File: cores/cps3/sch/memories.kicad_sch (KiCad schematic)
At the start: 2 parts, among them K12 29F016-90PFTN

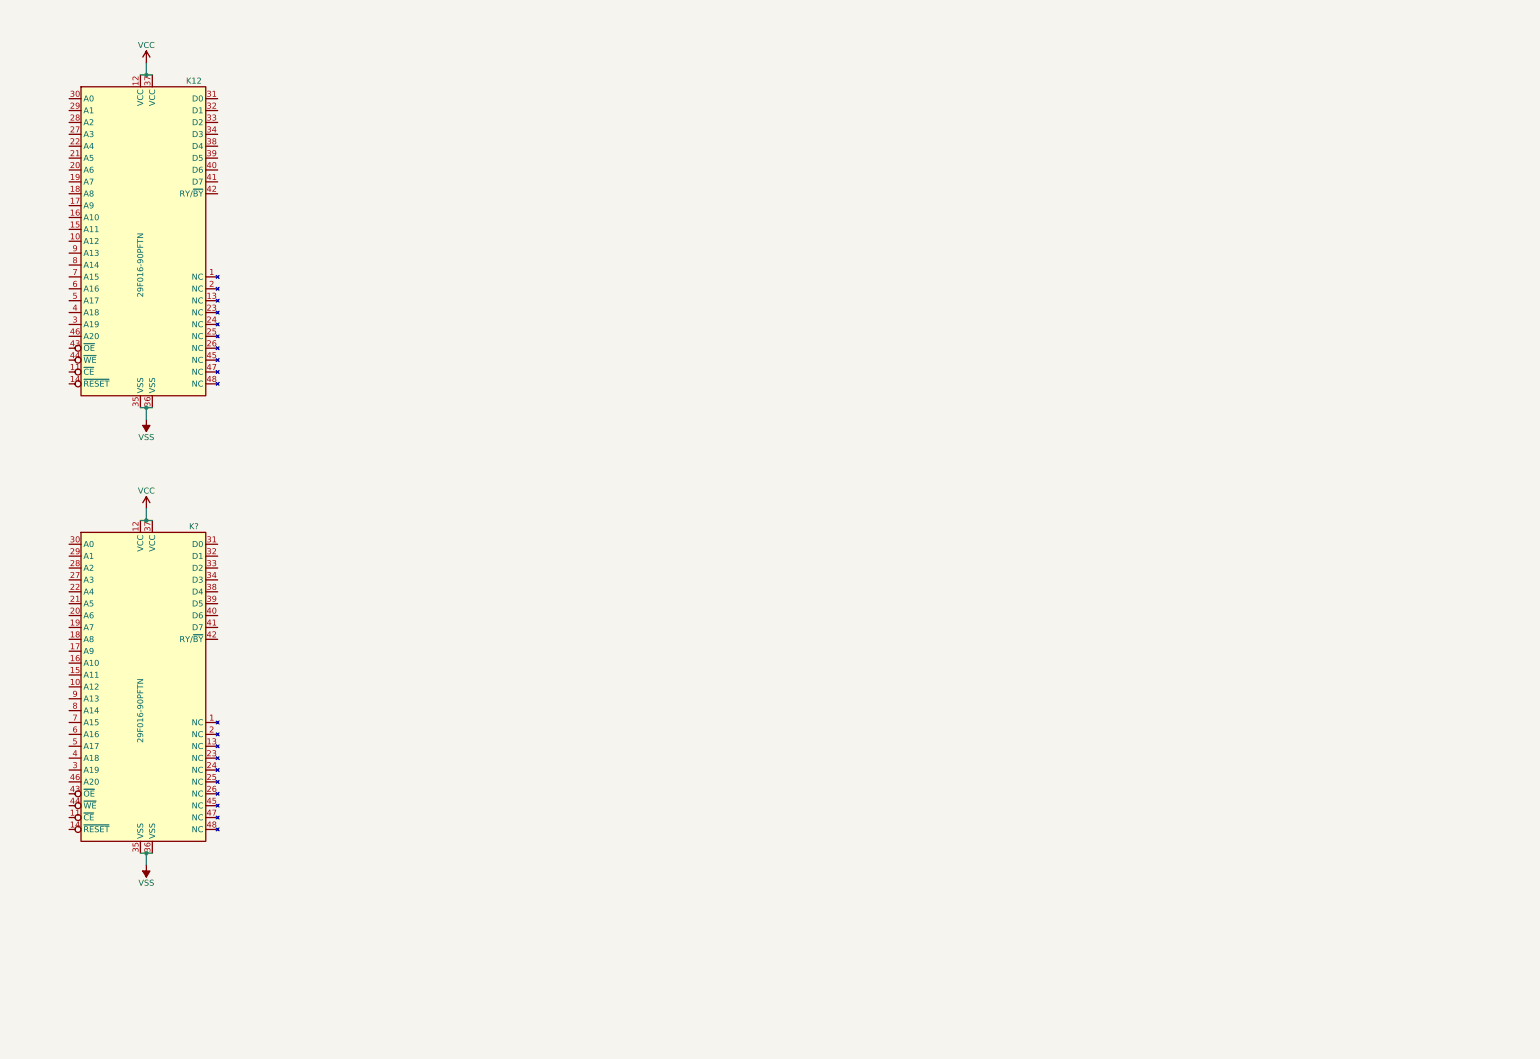
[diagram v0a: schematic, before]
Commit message: memories_gfx_main
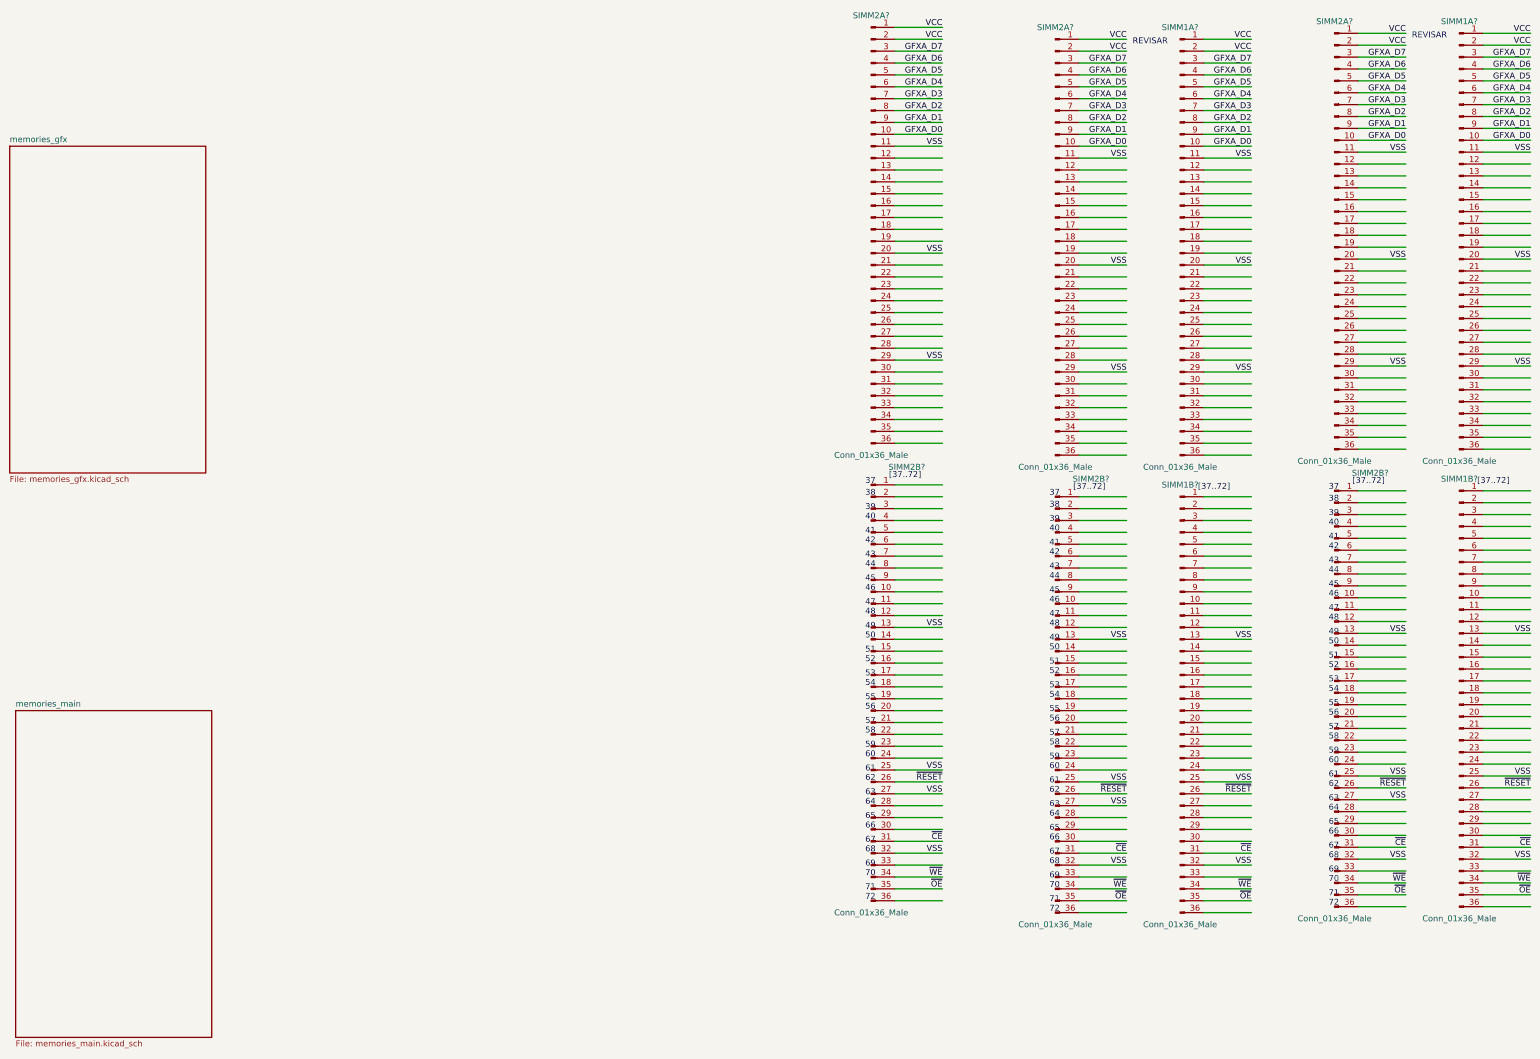
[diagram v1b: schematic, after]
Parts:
- removed K12, K?: 29F016-90PFTN, symbol arcade:29F016-90PFTN
- added SIMM1A? (x2), SIMM1B? (x2), SIMM2A? (x3), SIMM2B? (x3): Conn_01x36_Male, symbol Connector:Conn_01x36_Male
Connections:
- net VCC: now also SIMM1A?.1 (Pin_1), SIMM1A?.1 (Pin_1), SIMM1A?.2 (Pin_2), SIMM1A?.2 (Pin_2), SIMM2A?.1 (Pin_1), SIMM2A?.1 (Pin_1), SIMM2A?.1 (Pin_1), SIMM2A?.2 (Pin_2), SIMM2A?.2 (Pin_2), SIMM2A?.2 (Pin_2)
- net VSS: now also SIMM1A?.11 (Pin_11), SIMM1A?.11 (Pin_11), SIMM1A?.20 (Pin_20), SIMM1A?.20 (Pin_20), SIMM1A?.29 (Pin_29), SIMM1A?.29 (Pin_29), SIMM1B?.13 (Pin_13), SIMM1B?.13 (Pin_13), SIMM1B?.25 (Pin_25), SIMM1B?.25 (Pin_25), SIMM1B?.32 (Pin_32), SIMM1B?.32 (Pin_32), SIMM2A?.11 (Pin_11), SIMM2A?.11 (Pin_11), SIMM2A?.11 (Pin_11), SIMM2A?.20 (Pin_20), SIMM2A?.20 (Pin_20), SIMM2A?.20 (Pin_20), SIMM2A?.29 (Pin_29), SIMM2A?.29 (Pin_29), SIMM2A?.29 (Pin_29), SIMM2B?.13 (Pin_13), SIMM2B?.13 (Pin_13), SIMM2B?.13 (Pin_13), SIMM2B?.25 (Pin_25), SIMM2B?.25 (Pin_25), SIMM2B?.25 (Pin_25), SIMM2B?.27 (Pin_27), SIMM2B?.27 (Pin_27), SIMM2B?.27 (Pin_27), SIMM2B?.32 (Pin_32), SIMM2B?.32 (Pin_32), SIMM2B?.32 (Pin_32)
- new net GFXA_D0: SIMM1A?.10 (Pin_10), SIMM1A?.10 (Pin_10), SIMM2A?.10 (Pin_10), SIMM2A?.10 (Pin_10), SIMM2A?.10 (Pin_10)
- new net GFXA_D1: SIMM1A?.9 (Pin_9), SIMM1A?.9 (Pin_9), SIMM2A?.9 (Pin_9), SIMM2A?.9 (Pin_9), SIMM2A?.9 (Pin_9)
- new net GFXA_D2: SIMM1A?.8 (Pin_8), SIMM1A?.8 (Pin_8), SIMM2A?.8 (Pin_8), SIMM2A?.8 (Pin_8), SIMM2A?.8 (Pin_8)
- new net GFXA_D3: SIMM1A?.7 (Pin_7), SIMM1A?.7 (Pin_7), SIMM2A?.7 (Pin_7), SIMM2A?.7 (Pin_7), SIMM2A?.7 (Pin_7)
- new net GFXA_D4: SIMM1A?.6 (Pin_6), SIMM1A?.6 (Pin_6), SIMM2A?.6 (Pin_6), SIMM2A?.6 (Pin_6), SIMM2A?.6 (Pin_6)
- new net GFXA_D5: SIMM1A?.5 (Pin_5), SIMM1A?.5 (Pin_5), SIMM2A?.5 (Pin_5), SIMM2A?.5 (Pin_5), SIMM2A?.5 (Pin_5)
- new net GFXA_D6: SIMM1A?.4 (Pin_4), SIMM1A?.4 (Pin_4), SIMM2A?.4 (Pin_4), SIMM2A?.4 (Pin_4), SIMM2A?.4 (Pin_4)
- new net GFXA_D7: SIMM1A?.3 (Pin_3), SIMM1A?.3 (Pin_3), SIMM2A?.3 (Pin_3), SIMM2A?.3 (Pin_3), SIMM2A?.3 (Pin_3)
- new net ~{CE}: SIMM1B?.31 (Pin_31), SIMM1B?.31 (Pin_31), SIMM2B?.31 (Pin_31), SIMM2B?.31 (Pin_31), SIMM2B?.31 (Pin_31)
- new net ~{OE}: SIMM1B?.35 (Pin_35), SIMM1B?.35 (Pin_35), SIMM2B?.35 (Pin_35), SIMM2B?.35 (Pin_35), SIMM2B?.35 (Pin_35)
- new net ~{RESET}: SIMM1B?.26 (Pin_26), SIMM1B?.26 (Pin_26), SIMM2B?.26 (Pin_26), SIMM2B?.26 (Pin_26), SIMM2B?.26 (Pin_26)
- new net ~{WE}: SIMM1B?.34 (Pin_34), SIMM1B?.34 (Pin_34), SIMM2B?.34 (Pin_34), SIMM2B?.34 (Pin_34), SIMM2B?.34 (Pin_34)
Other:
- added sheet memories_gfx (memories_gfx.kicad_sch)
- added sheet memories_main (memories_main.kicad_sch)
- note added: "37"
- note added: "38"
- note added: "39 40"
- note added: "41 42"
- note added: "43 44"
- note added: "45 46"
- note added: "47 48"
- note added: "49 50"
- note added: "51 52"
- note added: "53 54"
- note added: "55 56"
- note added: "57 58"
- note added: "59 60"
- note added: "61 62"
- note added: "63 64"
- note added: "65 66"
- note added: "67 68"
- note added: "69 70"
- note added: "71 72"
- note added: "REVISAR"
- note added: "[37..72]"
